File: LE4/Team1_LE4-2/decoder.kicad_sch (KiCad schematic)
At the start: 4 parts, among them U16 74LS30, U17 74LS32, U18 74LS139, U19 74LS27

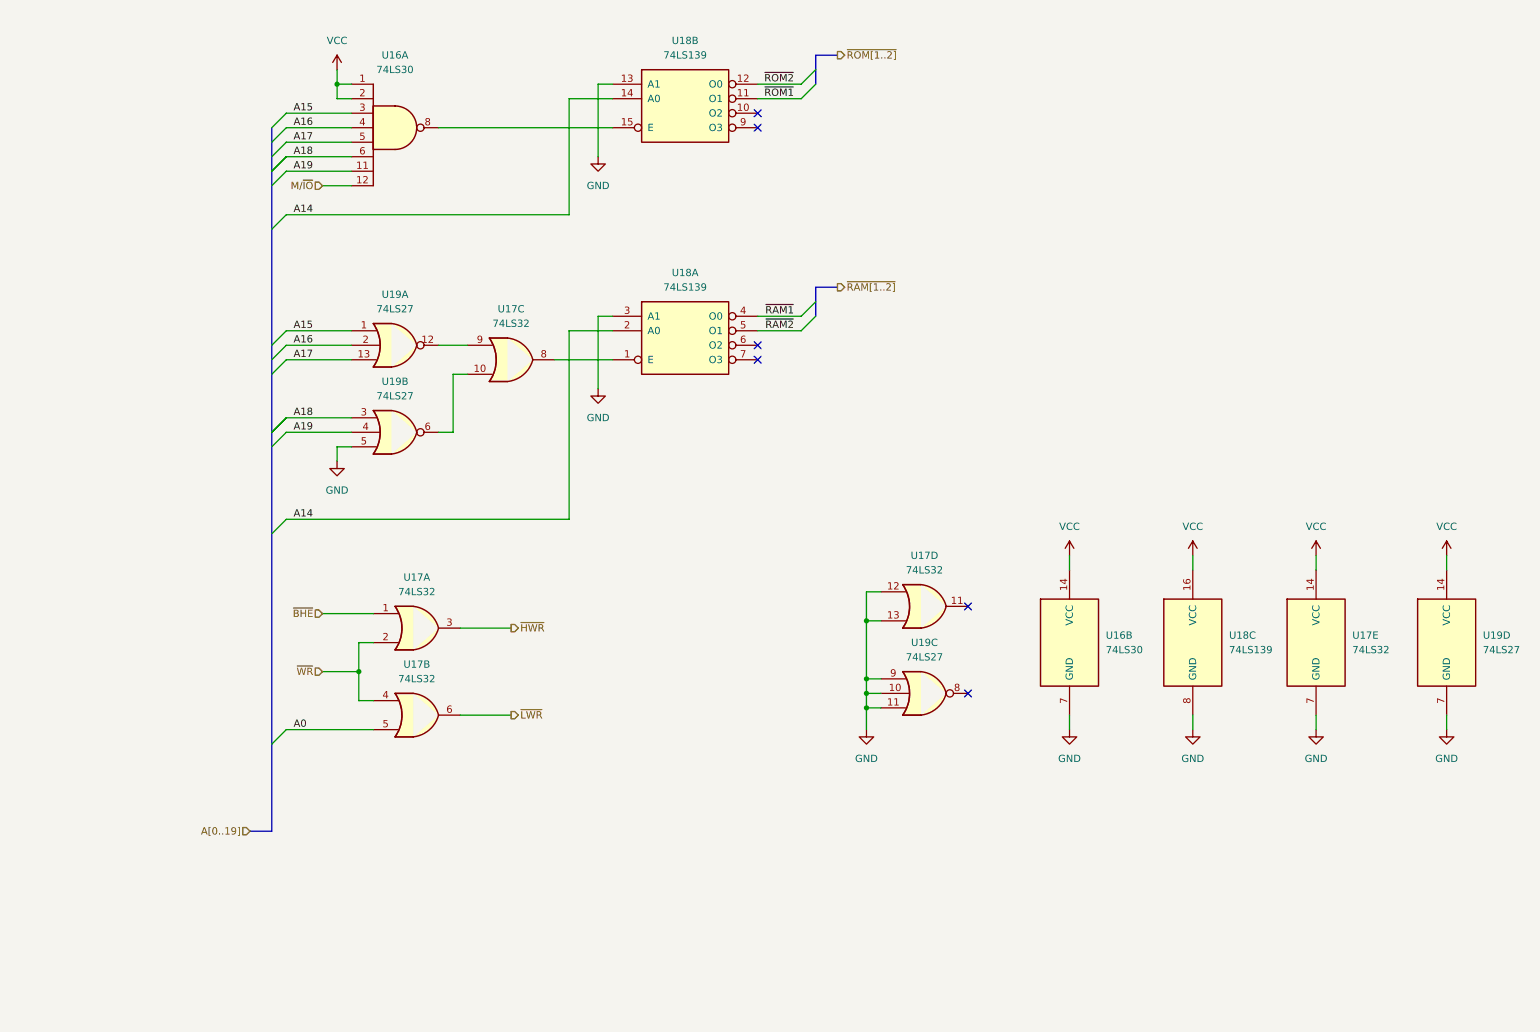
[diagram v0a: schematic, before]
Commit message: final updates to LE4-2
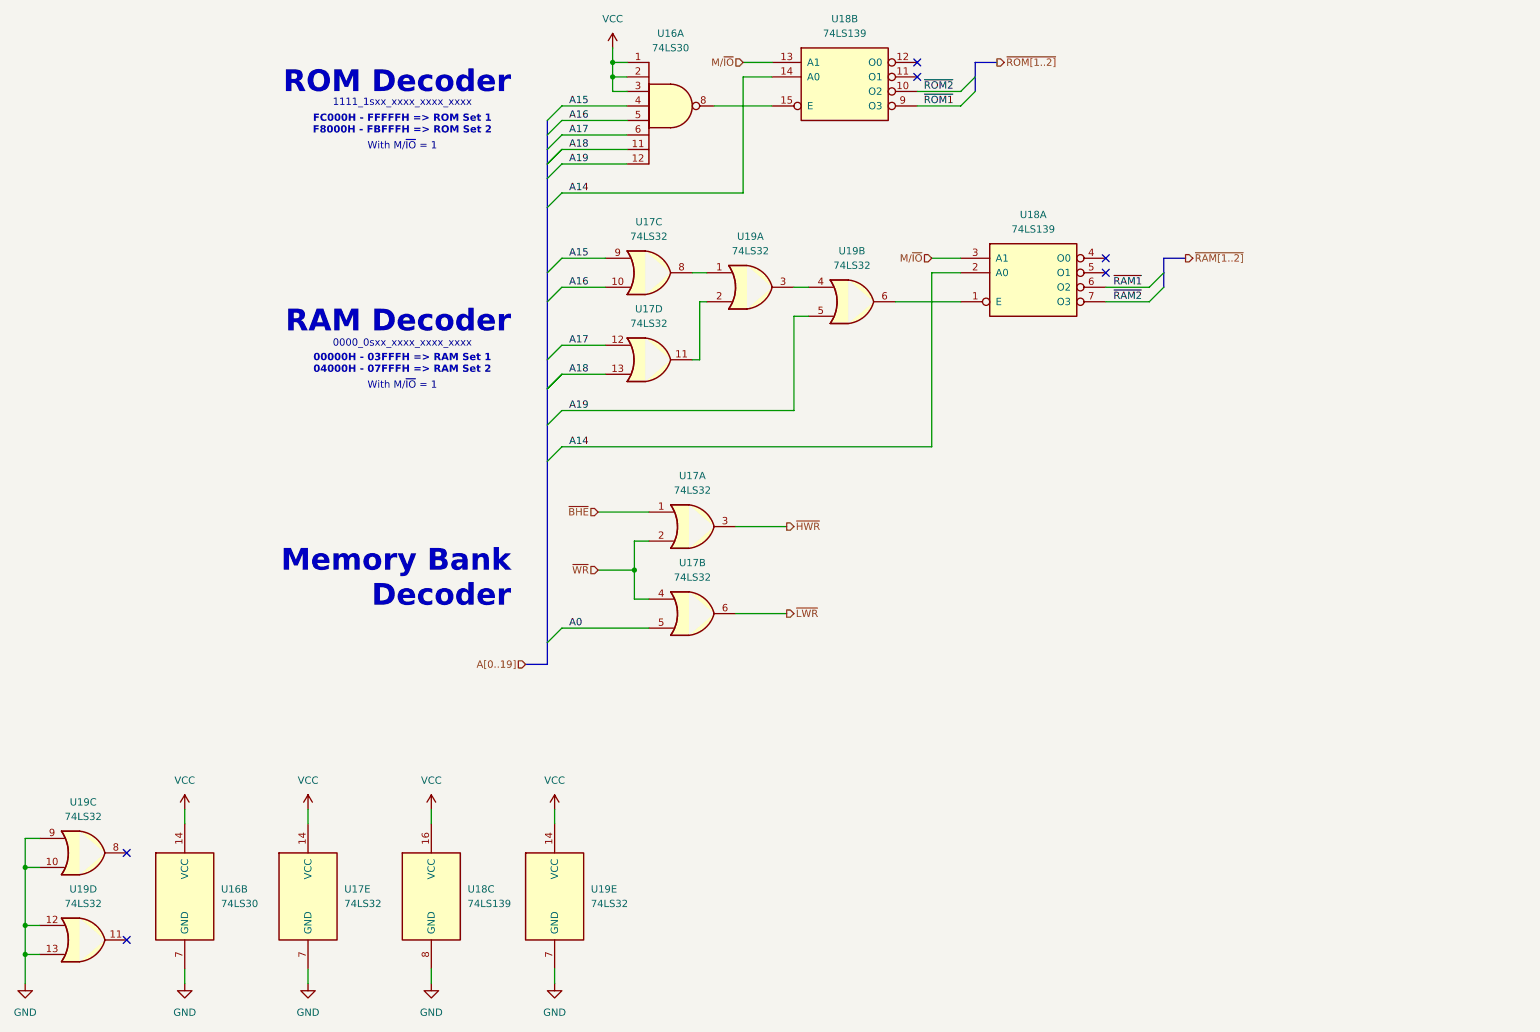
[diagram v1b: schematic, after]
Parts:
- removed U19: 74LS27, symbol 74xx:74LS27
- added U19: 74LS32, symbol 74xx:74LS32
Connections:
- net A15: now also U16.4, U17.9; no longer U16.3
- net A16: now also U16.5, U17.10; no longer U16.4
- net A17: now also U16.6, U17.12; no longer U16.5
- net A18: now also U16.11, U17.13; no longer U16.6
- net A19: now also U16.12, U19.5; no longer U16.11
- net GND: now also U19.10, U19.12, U19.13, U19.7 (GND), U19.9; no longer U17.12, U17.13, U18.13 (A1), U18.3 (A1)
- net M/~{IO}: now also U18.13 (A1), U18.3 (A1); no longer U16.12
- net VCC: now also U16.3, U19.14 (VCC)
- net ~{RAM1}: now also U18.6 (O2); no longer U18.4 (O0)
- net ~{RAM2}: now also U18.7 (O3); no longer U18.5 (O1)
- net ~{ROM1}: now also U18.9 (O3); no longer U18.11 (O1)
- net ~{ROM2}: now also U18.10 (O2); no longer U18.12 (O0)
- net at U17.11: now also U19.2
- net at U18.1 (E): now also U19.6; no longer U17.8
- new net: U19.3, U19.4
- new net: U17.8, U19.1
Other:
- note added: "00000H - 03FFFH => RAM Set 1 04000H - 07FFFH => RAM Set 2"
- note added: "0000_0sxx_xxxx_xxxx_xxxx"
- note added: "1111_1sxx_xxxx_xxxx_xxxx"
- note added: "FC000H - FFFFFH => ROM Set 1 F8000H - FBFFFH => ROM Set 2"
- note added: "Memory Bank Decoder"
- note added: "RAM Decoder"
- note added: "ROM Decoder"
- note added: "With M/~{IO} = 1"
- company: (none) -> Address Decoder sheet
- title: (none) -> Team1_LE4-2: Memory Interfacing (with Addressing Decoding)
- moved on the sheet: U16A, U16B, U17A, U17B, U17C, U17D, U17E, U18A, U18B, U18C
